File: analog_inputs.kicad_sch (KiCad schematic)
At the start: 34 parts, among them U201 74HC595

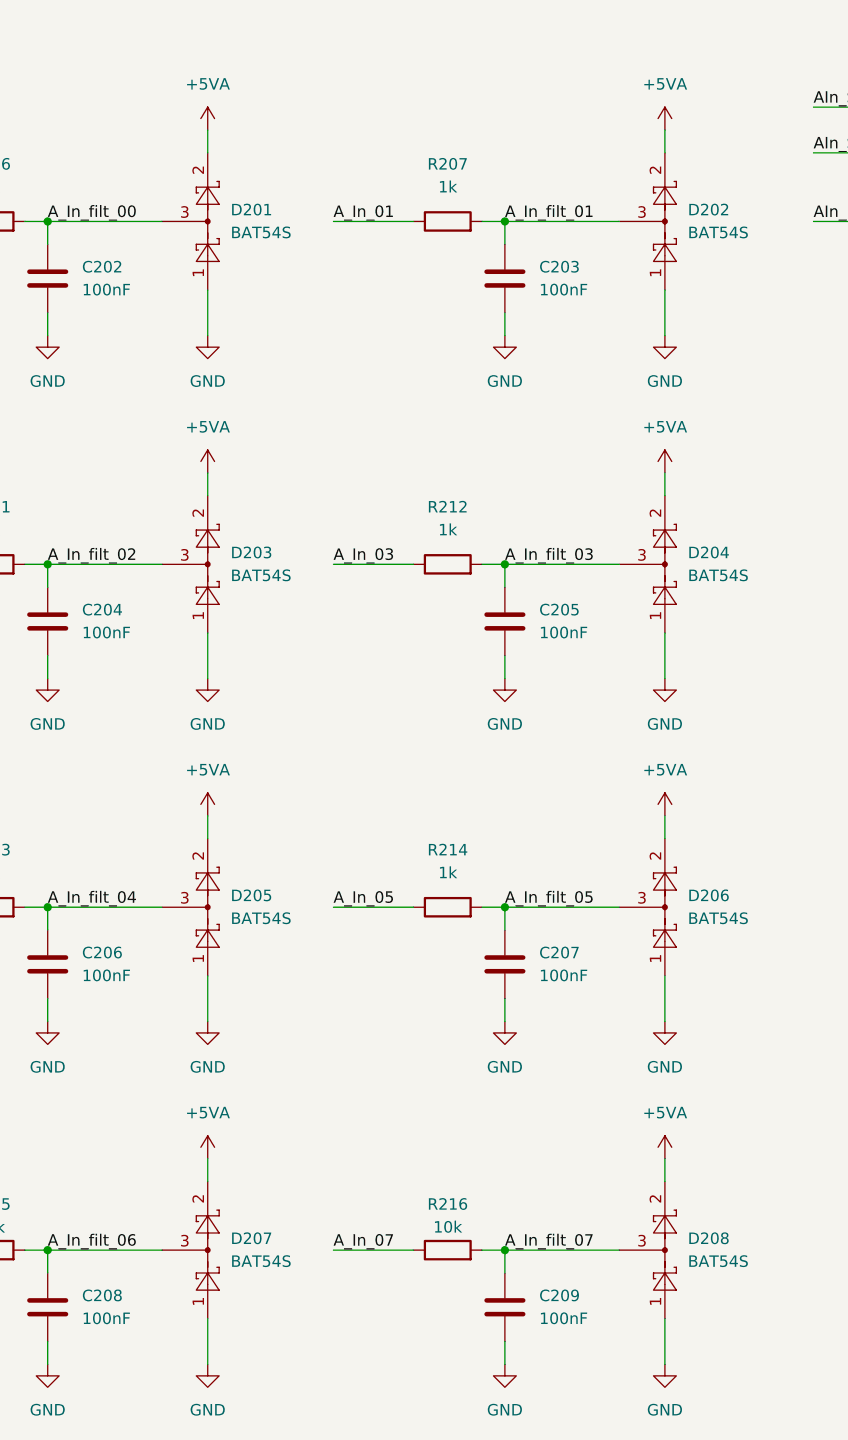
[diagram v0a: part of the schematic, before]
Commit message: completed schematic
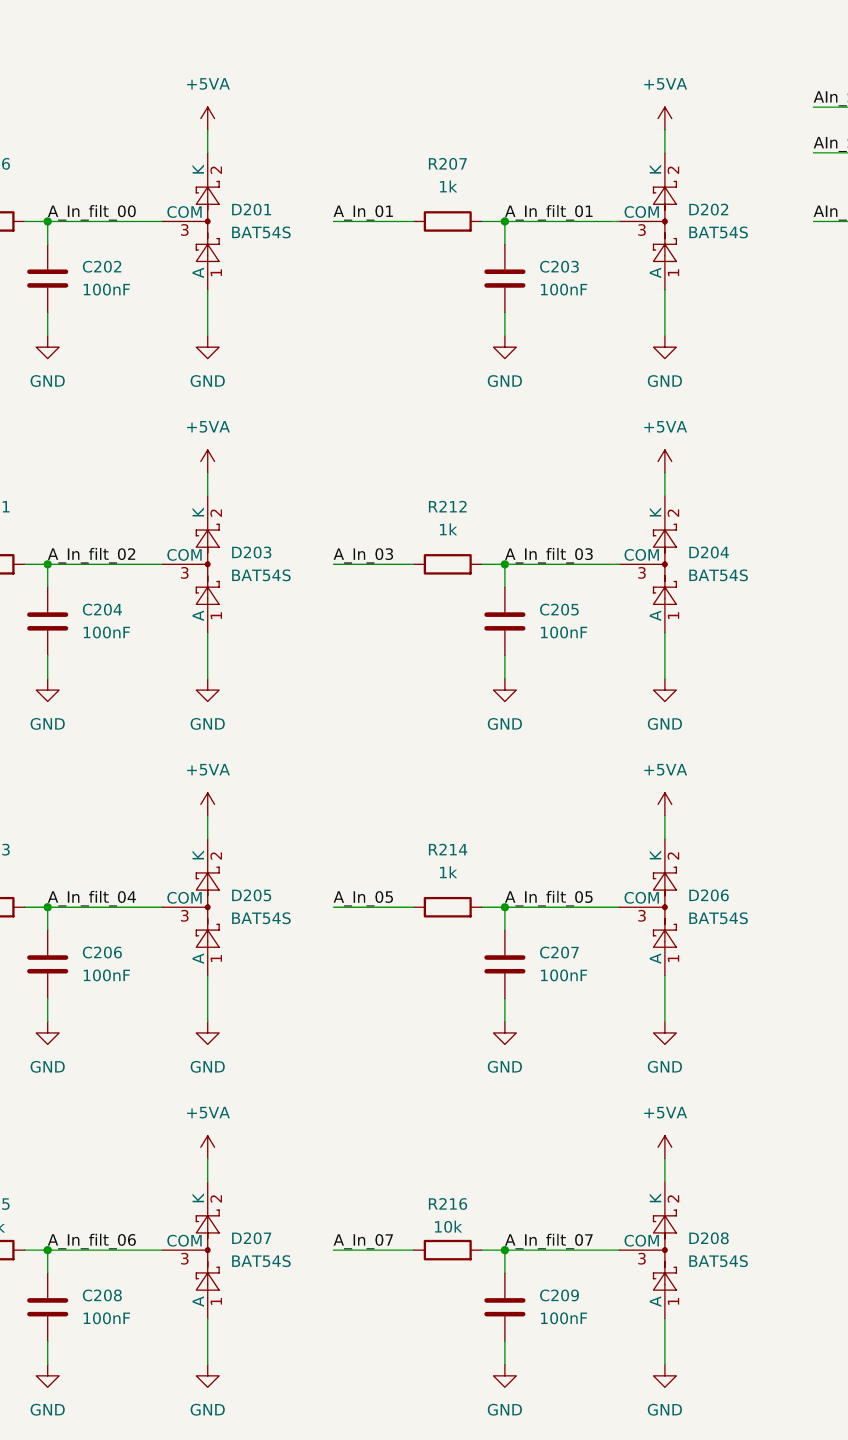
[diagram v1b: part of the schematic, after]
